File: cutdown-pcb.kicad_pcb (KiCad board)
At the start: 2 copper layers, 44.5 x 83.5 mm, 6 parts, among them J1 Conn_01x06

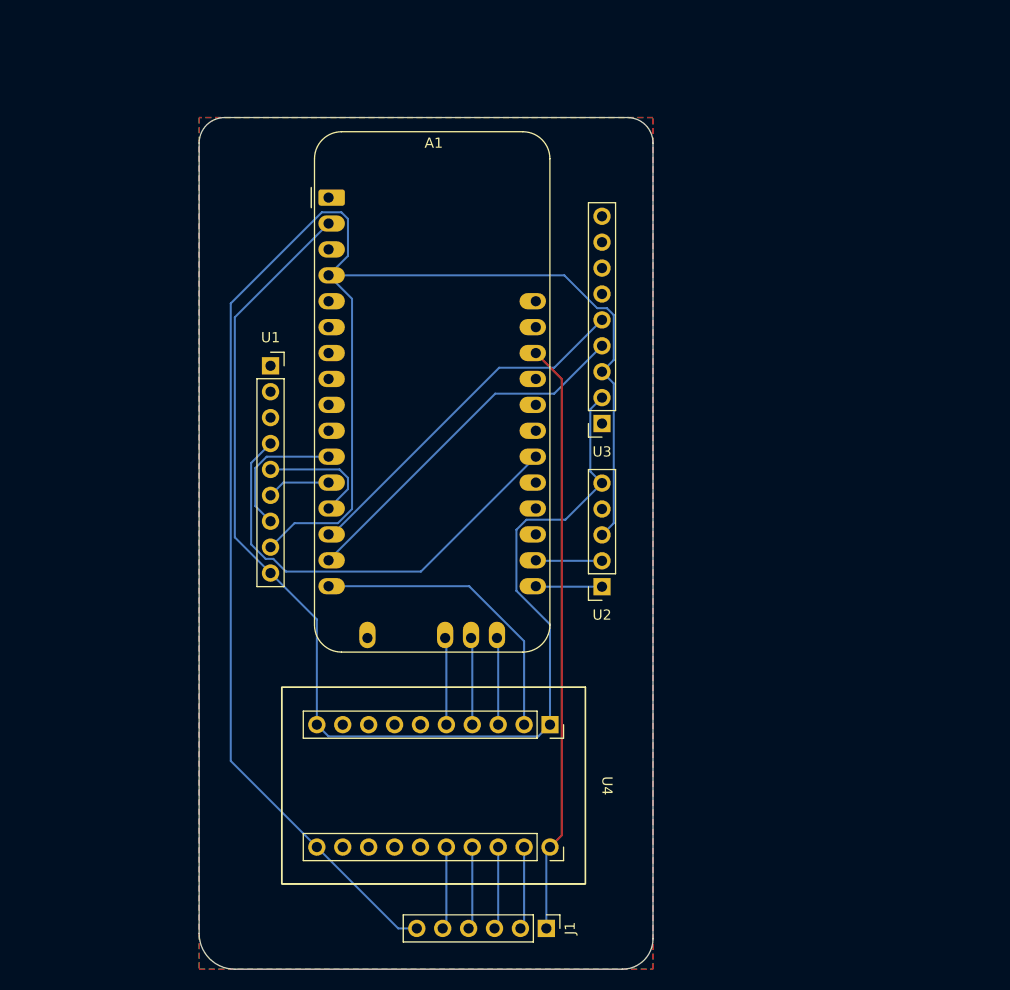
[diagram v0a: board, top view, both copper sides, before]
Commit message: Version 3
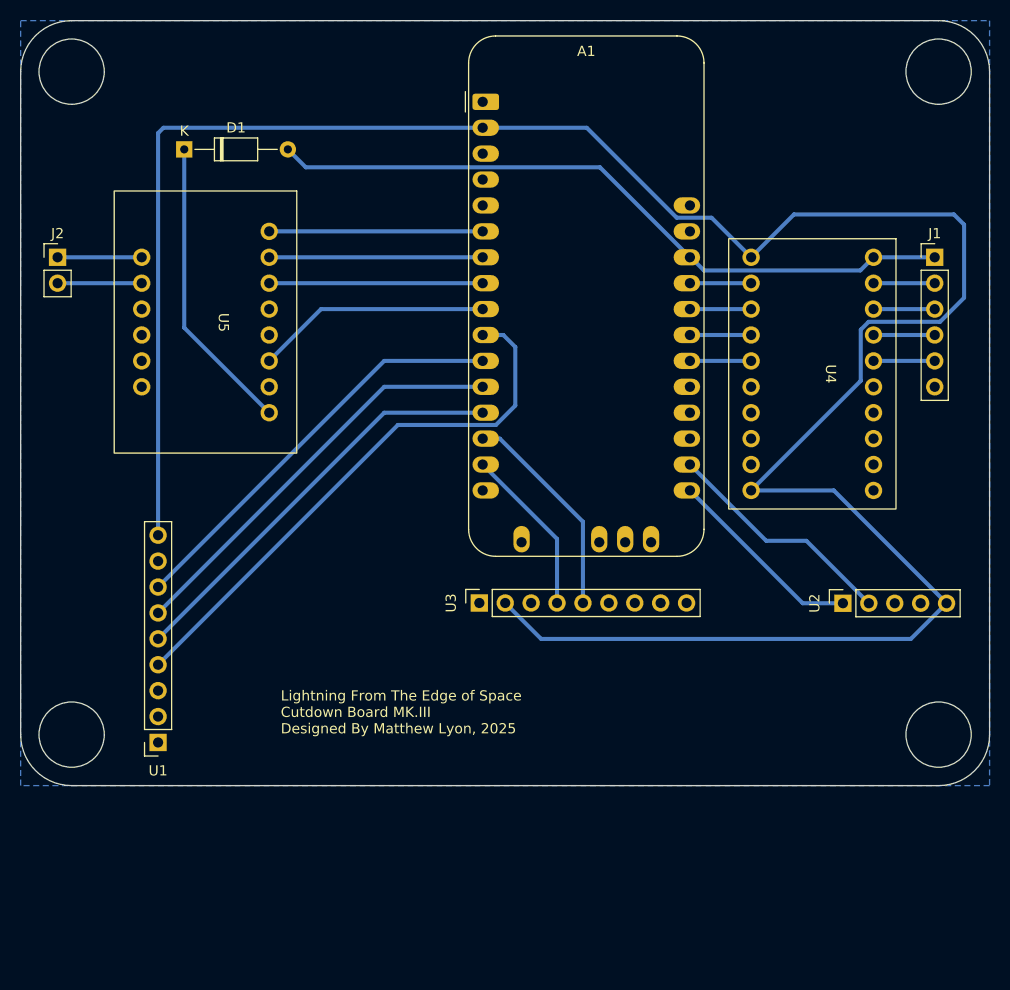
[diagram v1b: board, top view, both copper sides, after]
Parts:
- added D1: D, Diode_THT:D_DO-35_SOD27_P10.16mm_Horizontal, F.Cu at (116.0, 62.6)
- added J2: Conn_01x02_Pin, Connector_PinHeader_2.54mm:PinHeader_1x02_P2.54mm_Vertical, F.Cu at (103.6, 73.2)
- added U5: ~, CustomFootprints:AdafruitMotorDriverBreakout, F.Cu at (118.1, 79.5)
- moved J1 76.0 mm to (189.6, 73.2), turned to 0 degrees
- moved U4 54.8 mm to (177.6, 84.6)
- moved U1 38.5 mm to (113.5, 120.8), turned to 180 degrees
- moved U2 23.7 mm to (180.6, 107.1), turned to 90 degrees
- moved U3 21.3 mm to (145.0, 107.1), turned to 90 degrees
- moved A1 17.8 mm to (145.3, 58.0)
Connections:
- A1 pad 10: unconnected-(A1-A5-Pad10) -> Net-(A1-A5)
- A1 pad 16: /RL1 -> unconnected-(A1-DIO1-Pad16)
- A1 pad 21: unconnected-(A1-D9-Pad21) -> GND
- A1 pad 22: Net-(A1-D10) -> /RL4
- A1 pad 23: unconnected-(A1-D11-Pad23) -> /RL3
- A1 pad 24: unconnected-(A1-D12-Pad24) -> /RL2
- A1 pad 25: unconnected-(A1-D13-Pad25) -> /RL1
- A1 pad 30: /RL4 -> unconnected-(A1-DIO5-Pad30)
- A1 pad 31: /RL3 -> unconnected-(A1-DIO3-Pad31)
- A1 pad 32: /RL2 -> unconnected-(A1-DIO2-Pad32)
- A1 pad 6: unconnected-(A1-A1-Pad6) -> Net-(A1-A1)
- A1 pad 7: unconnected-(A1-A2-Pad7) -> Net-(A1-A2)
- A1 pad 8: unconnected-(A1-A3-Pad8) -> Net-(A1-A3)
- A1 pad 9: unconnected-(A1-A4-Pad9) -> Net-(A1-A4)
- U1 pad 4: Net-(A1-D10) -> Net-(A1-A5)
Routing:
- net GND: track 177.7 -> 0.00 mm
- net +3.3V: track 120.2 -> 234.8 mm
- net Net-(A1-A5): track 0.00 -> 55.0 mm
- net Net-(A1-D10): track 44.4 -> 0.00 mm
- net Net-(A1-MOSI/D23): track 6.21 -> 41.0 mm
- net Net-(A1-MISO/D22): track 11.7 -> 41.0 mm
- net Net-(D1-K): track 0.00 -> 29.3 mm
- net Net-(A1-SCK/D24): track 13.5 -> 41.0 mm
- net Net-(A1-A4): track 0.00 -> 23.0 mm
- net /RL1: track 29.6 -> 6.69 mm
- net Net-(A1-A3): track 0.00 -> 20.9 mm
- net Net-(A1-A2): track 0.00 -> 20.9 mm
- net Net-(A1-A1): track 0.00 -> 20.9 mm
- net Net-(A1-TX/D1): track 35.5 -> 16.6 mm
- net Net-(A1-SCL/D21): track 6.51 -> 23.3 mm
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- removed copper zone on F.Cu, net GND
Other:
- board size 44.5 x 83.5 mm -> 95 x 75 mm
- board text added: "Lightning From The Edge of Space Cutdown Board MK.III Designed By Matthew Lyon, 2025"
